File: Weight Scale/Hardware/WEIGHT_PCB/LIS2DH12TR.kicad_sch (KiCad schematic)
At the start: 3 parts, among them U2 LIS2DH12TR

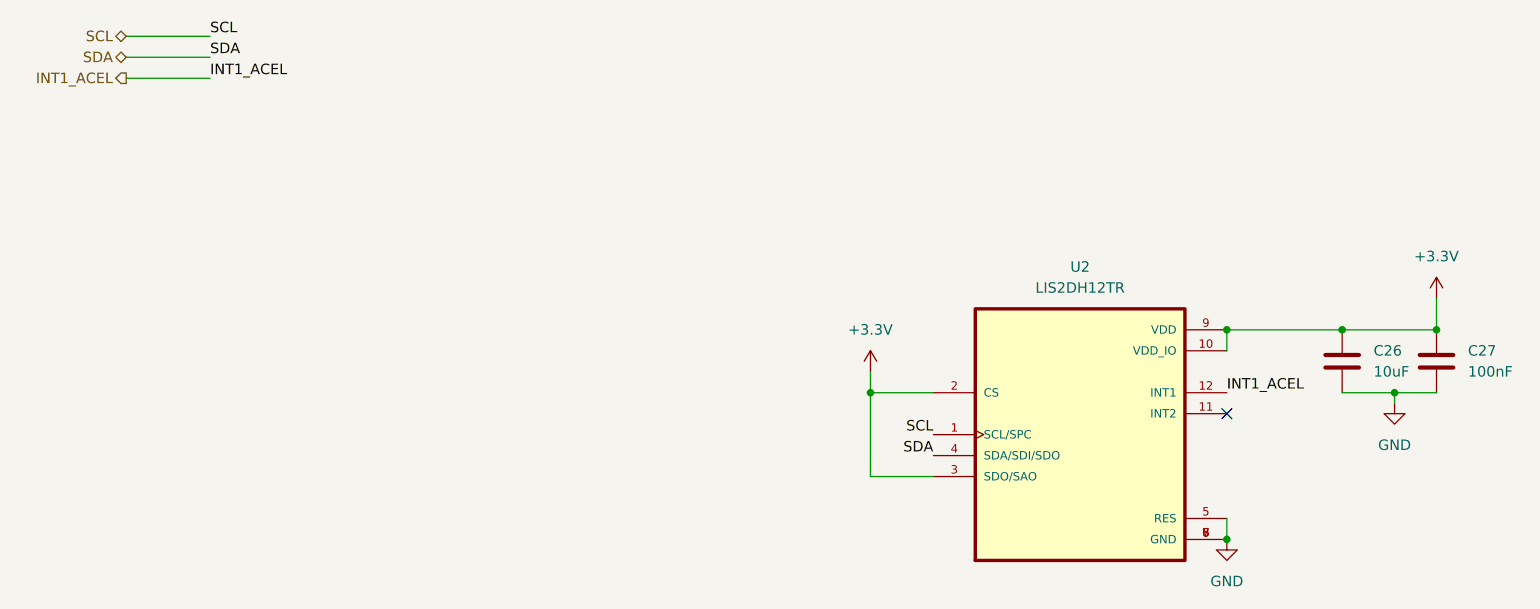
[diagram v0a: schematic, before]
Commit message: update schematics
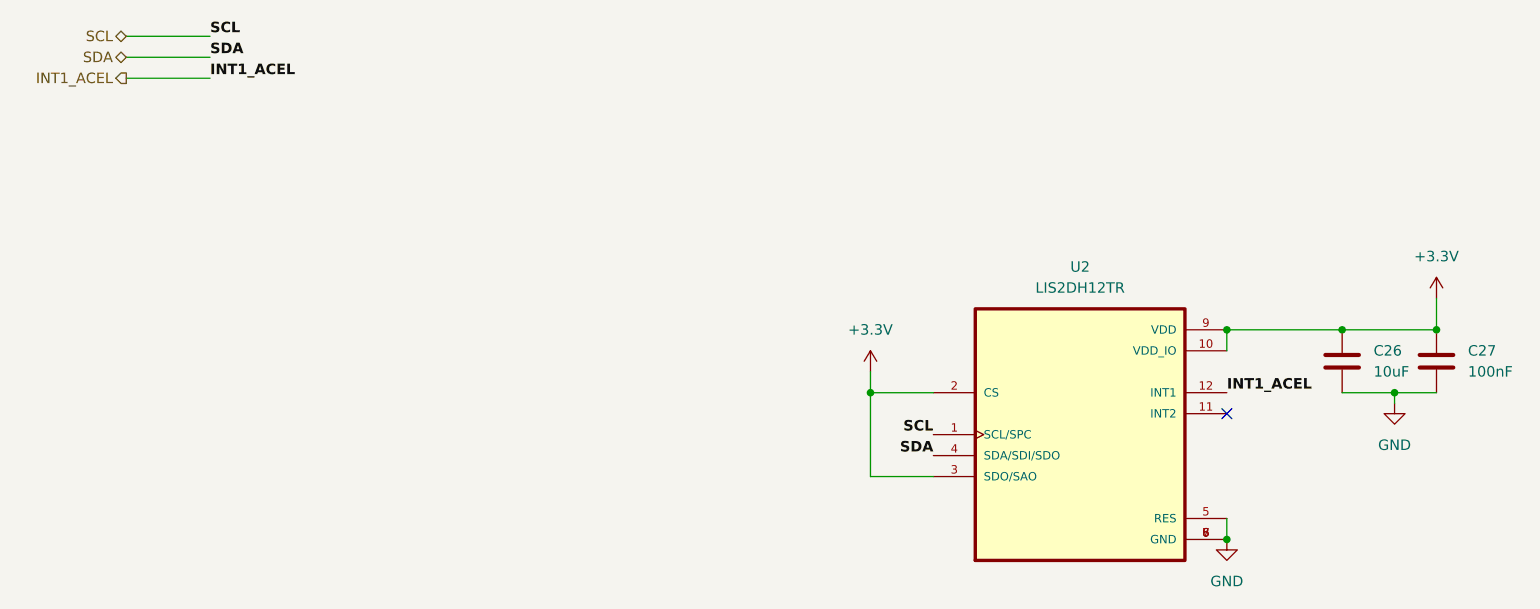
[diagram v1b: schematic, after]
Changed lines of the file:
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@@
 			(font
 				(size 1.27 1.27)
+				(bold yes)
 			)
 			(justify right bottom)
@@
 			(font
 				(size 1.27 1.27)
+				(bold yes)
 			)
 			(justify right bottom)
@@
 			(font
 				(size 1.27 1.27)
+				(bold yes)
 			)
 			(justify left bottom)
@@
 			(font
 				(size 1.27 1.27)
+				(bold yes)
 			)
 			(justify left bottom)
@@
 			(font
 				(size 1.27 1.27)
+				(bold yes)
 			)
 			(justify left bottom)
@@
 			(font
 				(size 1.27 1.27)
+				(bold yes)
 			)
 			(justify left bottom)
